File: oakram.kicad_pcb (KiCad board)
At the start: 2 copper layers, 4 parts, among them U1 IS41C16105C, U2 IS41C16105C, X1 ZIP40, X2 ZIP40

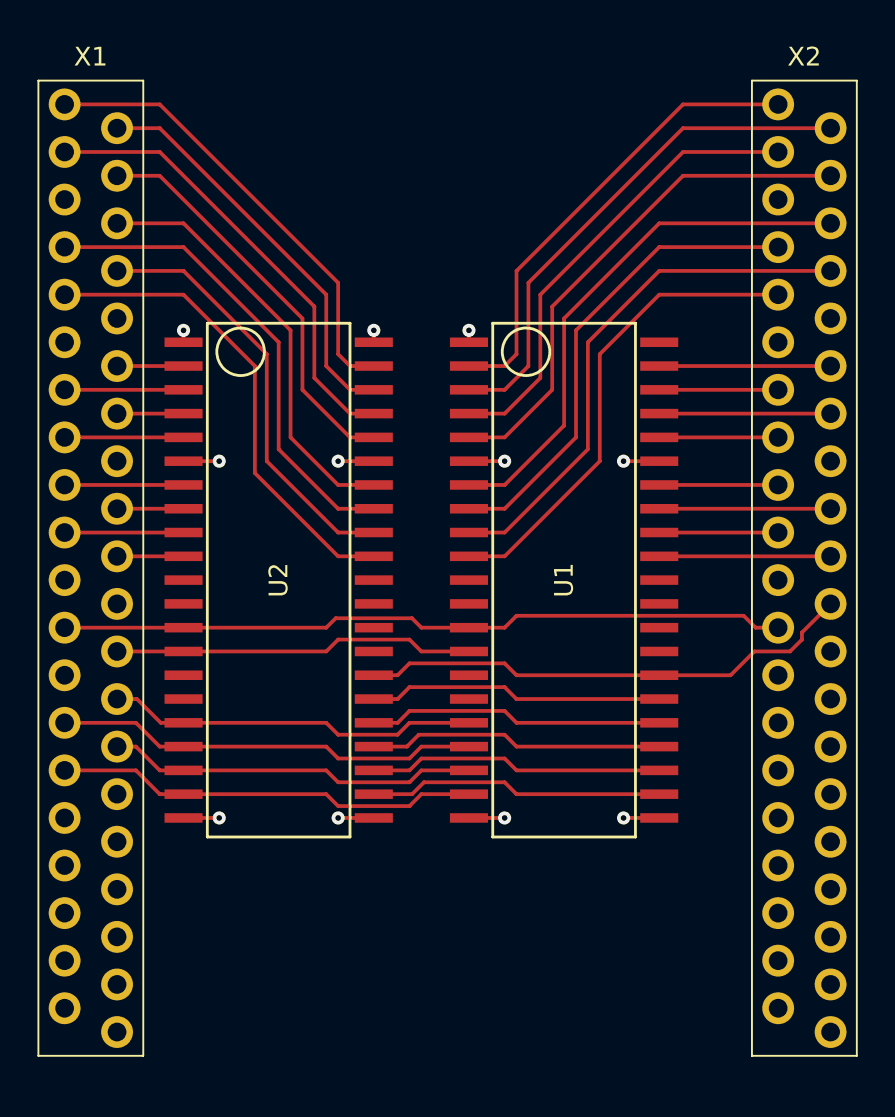
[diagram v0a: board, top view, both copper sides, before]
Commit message: Up
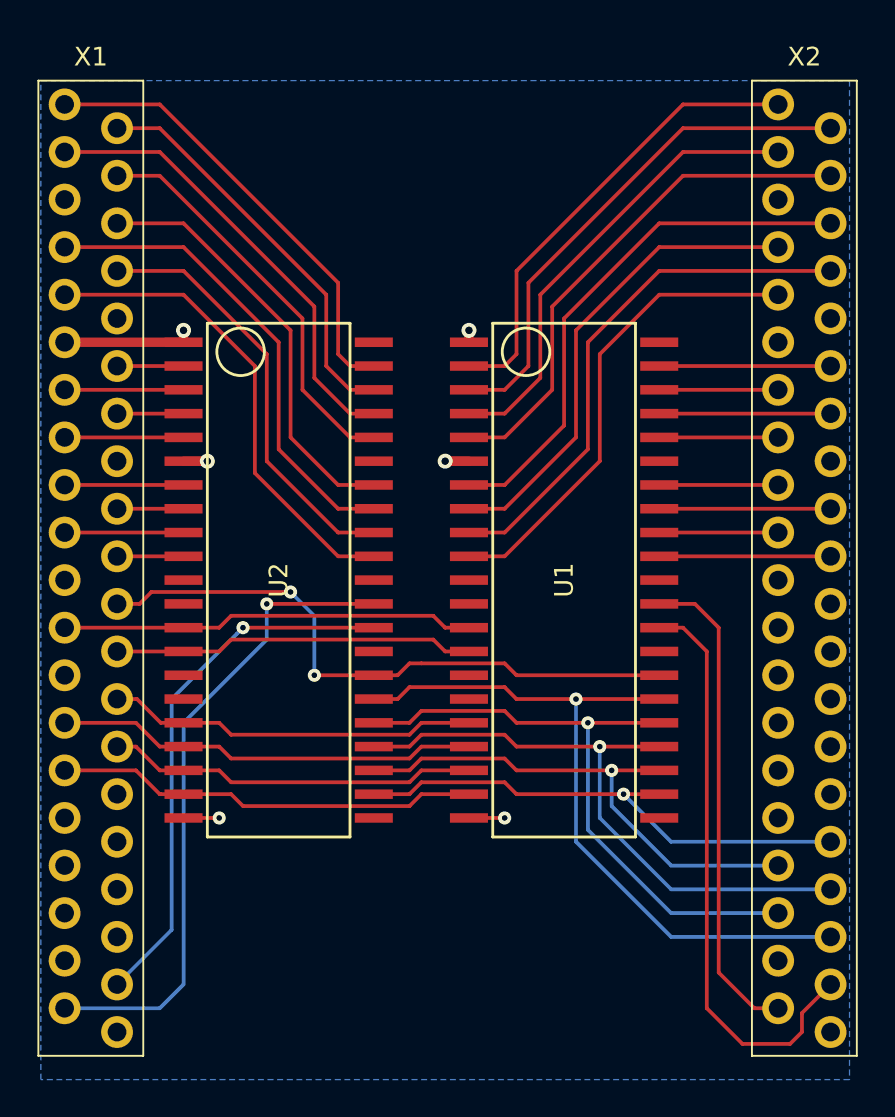
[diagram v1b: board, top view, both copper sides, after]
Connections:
- X1 pad 32: /A4 -> Net-(X1-Pad32)
- X1 pad 33: /A5 -> Net-(X1-Pad33)
- X1 pad 34: /A6 -> Net-(X1-Pad34)
- X1 pad 35: /A7 -> Net-(X1-Pad35)
- X1 pad 36: /A8 -> Net-(X1-Pad36)
- X2 pad 22: /A9 -> Net-(X2-Pad22)
- X2 pad 23: /~WE -> Net-(X2-Pad23)
- X2 pad 24: /~RAS -> Net-(X2-Pad24)
- X2 pad 26: /A0 -> Net-(X2-Pad26)
- X2 pad 27: /A1 -> Net-(X2-Pad27)
- X2 pad 28: /A2 -> Net-(X2-Pad28)
- X2 pad 29: /A3 -> Net-(X2-Pad29)
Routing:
- net /~CAS0: track 0.00 -> 34.8 mm, vias 0 -> 1
- net /~CAS3: track 0.00 -> 31.4 mm
- net /~CAS1: track 0.00 -> 28.8 mm, vias 0 -> 1
- net /~CAS2: track 0.00 -> 26.1 mm
- net /A8: track 15.8 -> 39.1 mm, vias 0 -> 1
- net /A7: track 15.8 -> 33.5 mm, vias 0 -> 1
- net /A6: track 15.8 -> 33.5 mm, vias 0 -> 1
- net /~WE: track 39.0 -> 22.1 mm
- net /A5: track 15.8 -> 27.9 mm, vias 0 -> 1
- net /A4: track 15.8 -> 27.9 mm, vias 0 -> 1
- net VSS: track 8.26 -> 0.00 mm, vias 5 -> 0
- net /A9: track 26.7 -> 33.4 mm, vias 0 -> 2
- net VCC: track 8.89 -> 14.0 mm
- added copper zone on B.Cu, net GND
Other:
- net class Default: via_dia 0.7 -> 0.8; via_drill 0.3 -> 0.4
- rule via_min_drill: 0.3 -> 0.4
- rule via_min_size: 0.4 -> 0.8
